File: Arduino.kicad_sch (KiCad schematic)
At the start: 14 parts

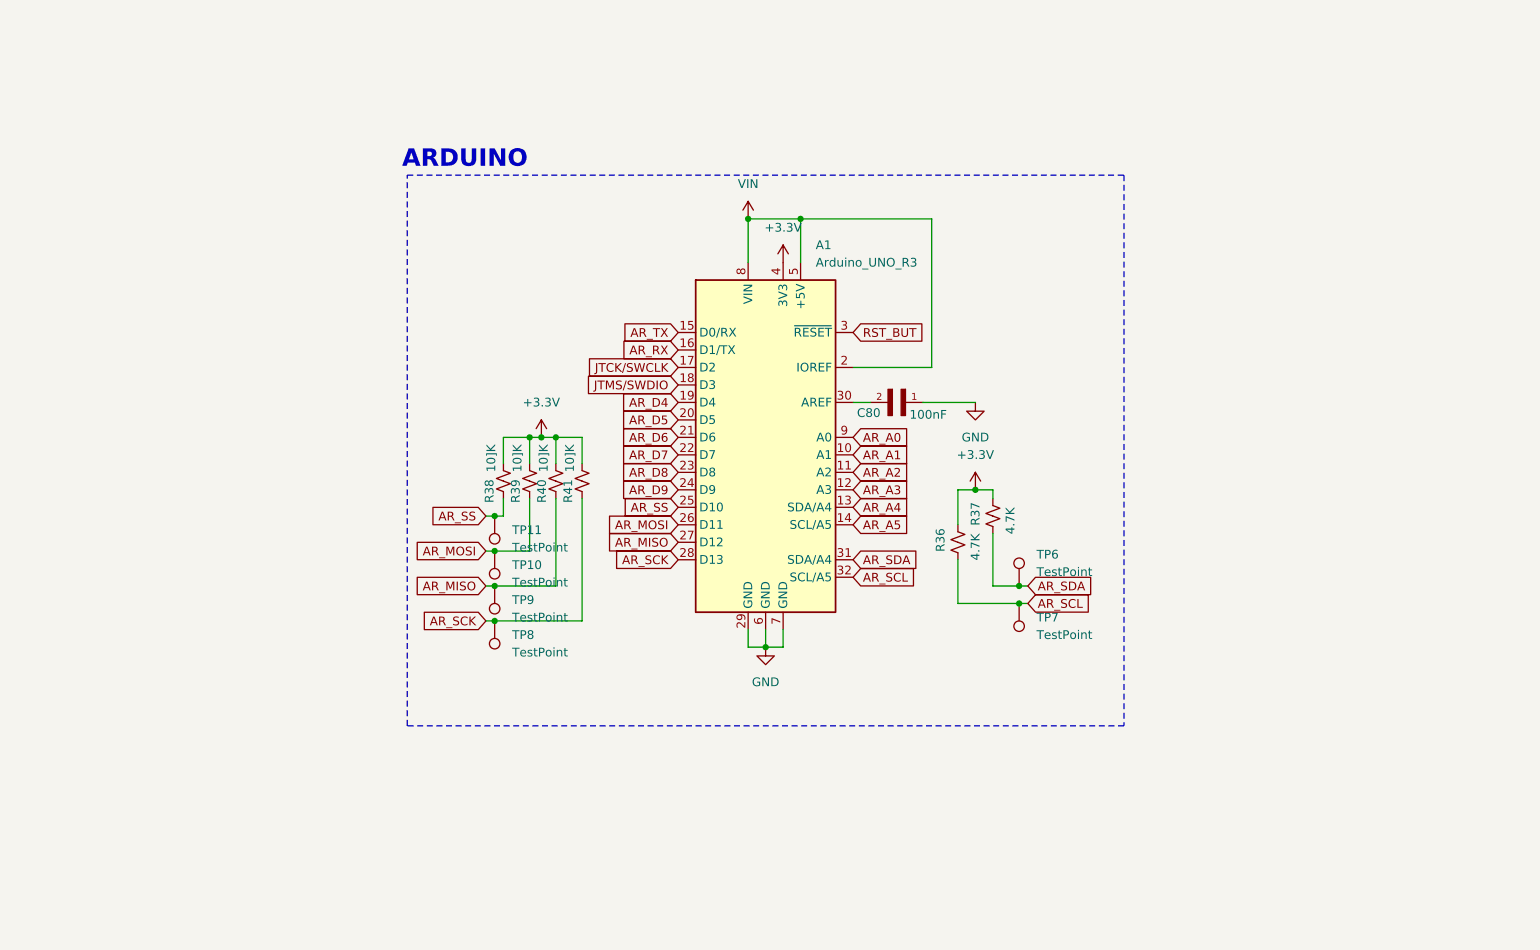
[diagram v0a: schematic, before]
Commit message: new
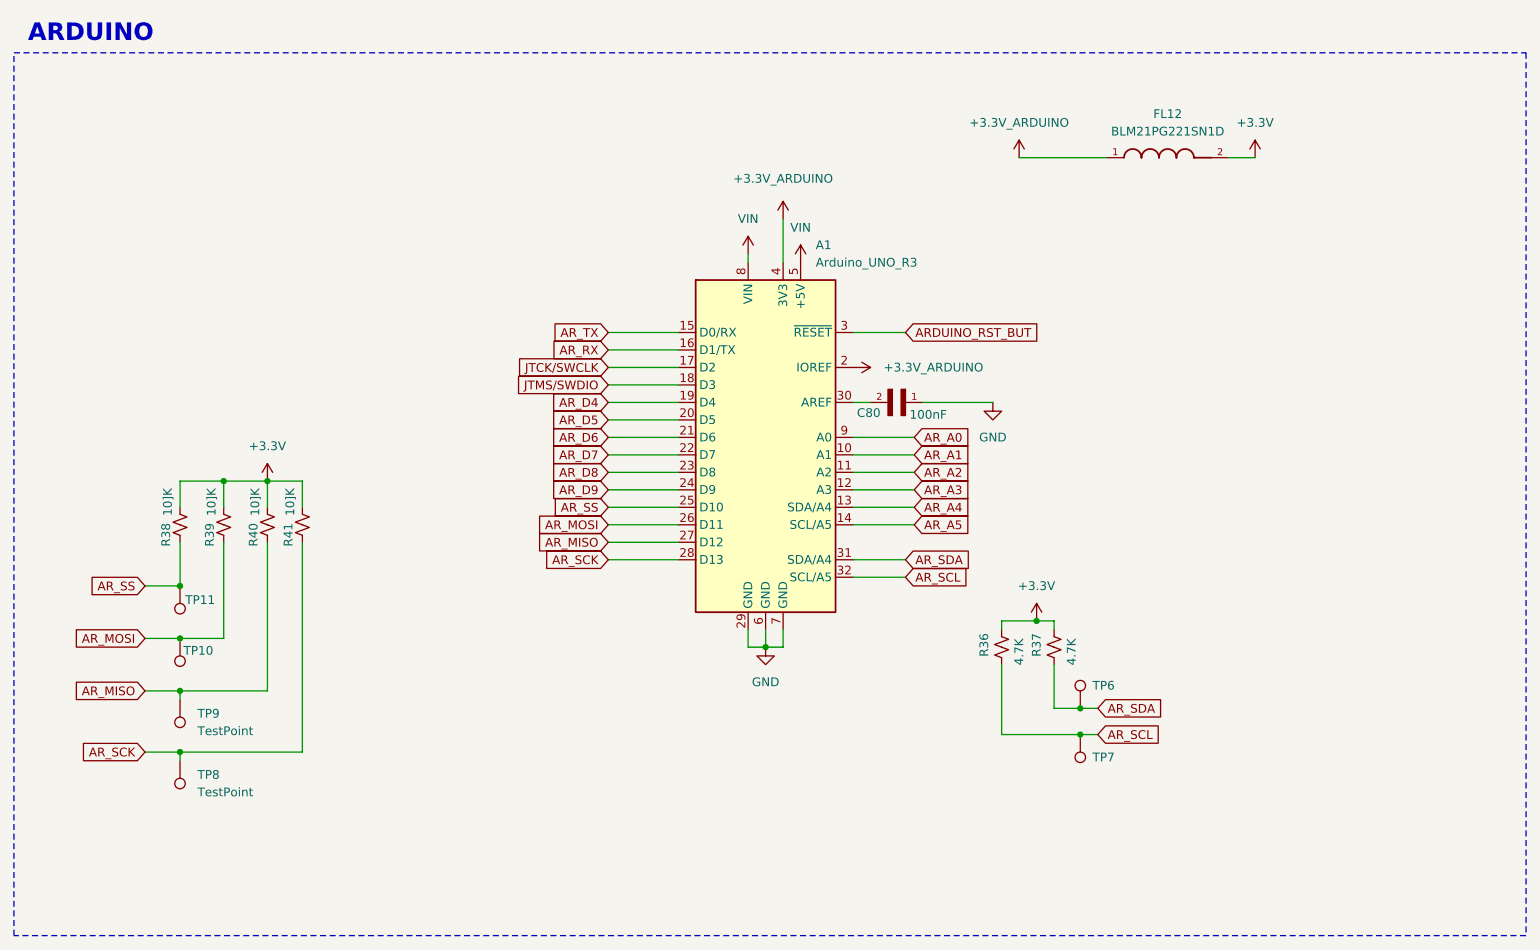
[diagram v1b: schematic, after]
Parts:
- added FL12: BLM21PG221SN1D, BLM21PG221SN1D:BEADC2012X105N, symbol BLM21PG221SN1D:BLM21PG221SN1D
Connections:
- net +3.3V: now also FL12.2; no longer A1.4 (3V3)
- net VIN: no longer A1.2 (IOREF)
- net RST_BUT renamed ARDUINO_RST_BUT
- new net +3.3V_ARDUINO: A1.2 (IOREF), A1.4 (3V3), FL12.1
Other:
- moved on the sheet: R36, R37, R38, R39, R40, R41, TP10, TP11, TP6, TP7, TP8, TP9
